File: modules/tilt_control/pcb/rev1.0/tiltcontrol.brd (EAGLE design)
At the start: 50 x 36.5 mm, 25 parts, among them IC1 PICAXE-08M2, IC2 PICAXE-08M2, IC3 BD6211F-E2, J1 Potentiometer

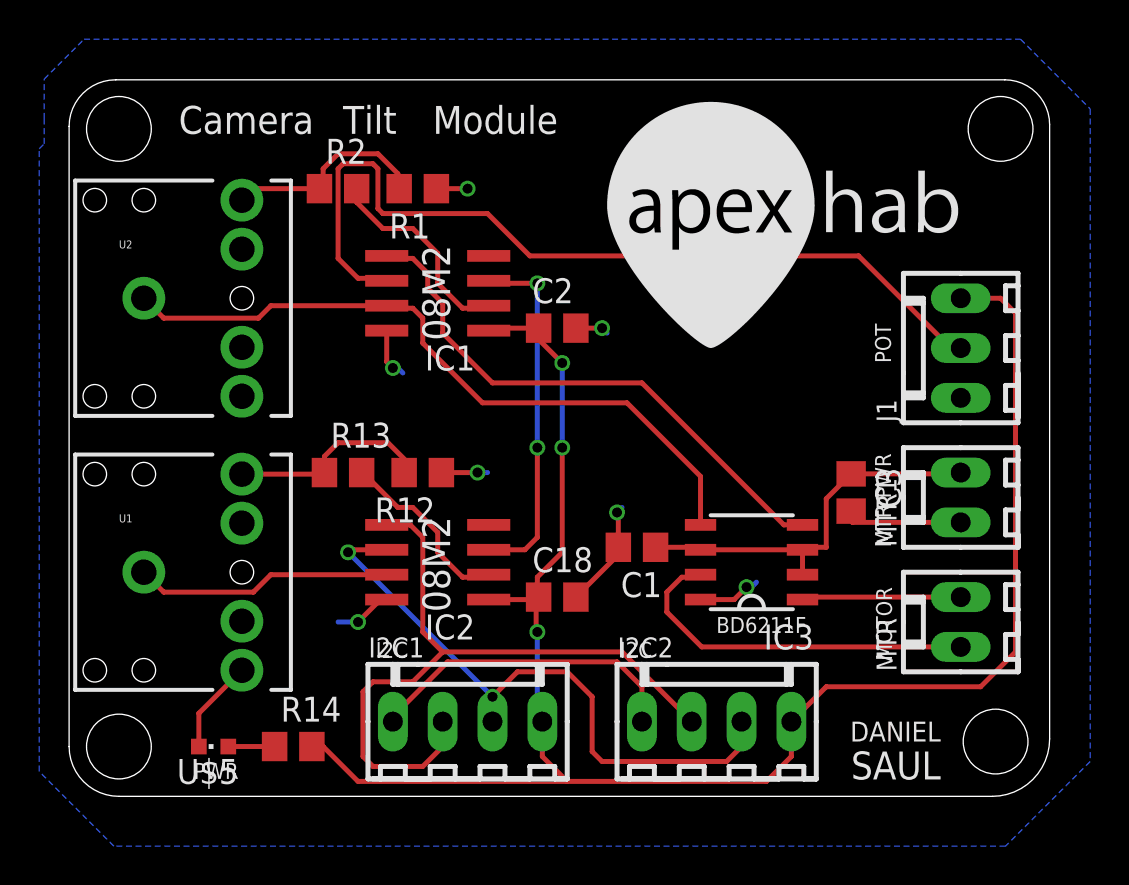
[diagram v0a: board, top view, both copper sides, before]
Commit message: fix airwires, rename, export larger pngs
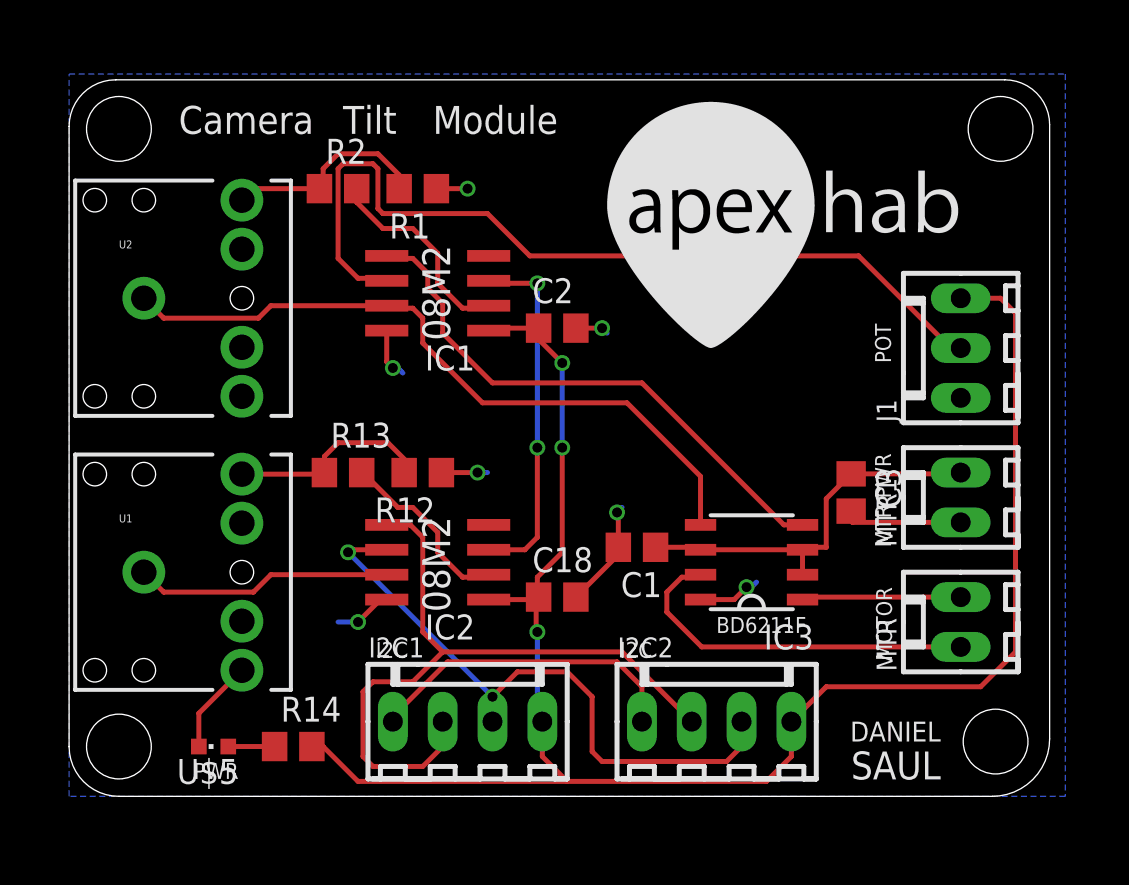
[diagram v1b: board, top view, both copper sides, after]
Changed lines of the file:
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@@
 <setting verticaltext="up"/>
 </settings>
-<grid distance="0.01" unitdist="inch" unit="inch" style="lines" multiple="1" display="yes" altdistance="0.005" altunitdist="inch" altunit="inch"/>
+<grid distance="0.05" unitdist="inch" unit="inch" style="lines" multiple="1" display="yes" altdistance="0.005" altunitdist="inch" altunit="inch"/>
 <layers>
 <layer number="1" name="Top" color="4" fill="1" visible="yes" active="yes"/>
@@
 <wire x1="45.466" y1="13.97" x2="39.944" y2="13.97" width="0.254" layer="1"/>
 <wire x1="39.944" y1="13.97" x2="39.878" y2="14.544" width="0.254" layer="1"/>
-<polygon width="0.254" layer="16" isolate="0.254">
-<vertex x="-1.27" y="34.544"/>
-<vertex x="-1.27" y="36.576"/>
-<vertex x="0.762" y="38.608"/>
-<vertex x="48.514" y="38.608"/>
-<vertex x="52.07" y="35.052"/>
-<vertex x="52.07" y="1.778"/>
-<vertex x="47.752" y="-2.54"/>
-<vertex x="2.286" y="-2.54"/>
-<vertex x="-1.524" y="1.27"/>
-<vertex x="-1.524" y="33.02"/>
-<vertex x="-1.27" y="33.274"/>
-</polygon>
 <wire x1="18.73" y1="30.988" x2="20.32" y2="30.988" width="0.254" layer="1"/>
 <via x="20.32" y="30.988" extent="1-16" drill="0.508"/>
@@
 <wire x1="34.544" y1="10.668" x2="34.798" y2="10.668" width="0.254" layer="16"/>
 <wire x1="34.798" y1="10.668" x2="35.052" y2="10.922" width="0.254" layer="16"/>
+<polygon width="0.254" layer="16" isolate="0.254">
+<vertex x="0" y="36.83"/>
+<vertex x="50.8" y="36.83"/>
+<vertex x="50.8" y="0"/>
+<vertex x="0" y="0"/>
+</polygon>
 </signal>
 <signal name="SCL">
@@
 <contactref element="U2" pad="RING"/>
 <wire x1="12.766" y1="30.988" x2="12.766" y2="31.562" width="0.254" layer="1"/>
-<wire x1="16.764" y1="31.75" x2="16.764" y2="30.988" width="0.254" layer="1"/>
 <wire x1="12.766" y1="30.988" x2="9.398" y2="30.988" width="0.254" layer="1"/>
 <wire x1="9.398" y1="30.988" x2="8.81" y2="30.4" width="0.254" layer="1"/>
-<wire x1="16.764" y1="31.75" x2="15.748" y2="32.766" width="0.254" layer="1"/>
 <wire x1="15.748" y1="32.766" x2="13.716" y2="32.766" width="0.254" layer="1"/>
 <wire x1="13.716" y1="32.766" x2="12.954" y2="32.004" width="0.254" layer="1"/>
 <wire x1="12.954" y1="32.004" x2="12.954" y2="31.176" width="0.254" layer="1"/>
 <wire x1="12.954" y1="31.176" x2="12.766" y2="30.988" width="0.254" layer="1"/>
-<wire x1="16.764" y1="30.988" x2="16.83" y2="30.988" width="0" layer="19" extent="1-1"/>
+<wire x1="16.83" y1="30.988" x2="16.83" y2="31.684" width="0.254" layer="1"/>
+<wire x1="16.83" y1="31.684" x2="15.748" y2="32.766" width="0.254" layer="1"/>
 </signal>
 <signal name="SER">
